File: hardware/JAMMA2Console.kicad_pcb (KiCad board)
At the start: 4 copper layers, 126 x 131.5 mm, 212 parts, among them J1 Conn_02x28_JAMMA, J10 Conn_02x03_Odd_Even, J11 Conn_02x05_Odd_Even, J12 Conn_01x03, J13 Conn_01x03, J2 DS1038-15FBNSiA74-0CC, J3 SCART-F, J4 DF1BZ-34DP-2.5DSA, J5 PJ-320D, J6 DS1037-15FNAKT74-0CC, J7 DS1037-15FNAKT74-0CC, J8 Phoenix PTS 1,5/4-5.0, J9 Molex 67503-1020, SW1 SW_Push, SW2 SW_Push, SW3 SW_Push, U1 USBLC6-2P6, U10 74LVC4245, U11 74LVC4245, U13 PAM8610, U14 PAM8610, U15 74HCT4053, U16 STM32F103VCT6, U2 LD1117-3.3, U3 74HCT4053, U4 74HCT86, U5 74HCT4053, U6 LM1881, U7 THS7375, U8 TL072, U9 74LVC4245, Y1 12MHz

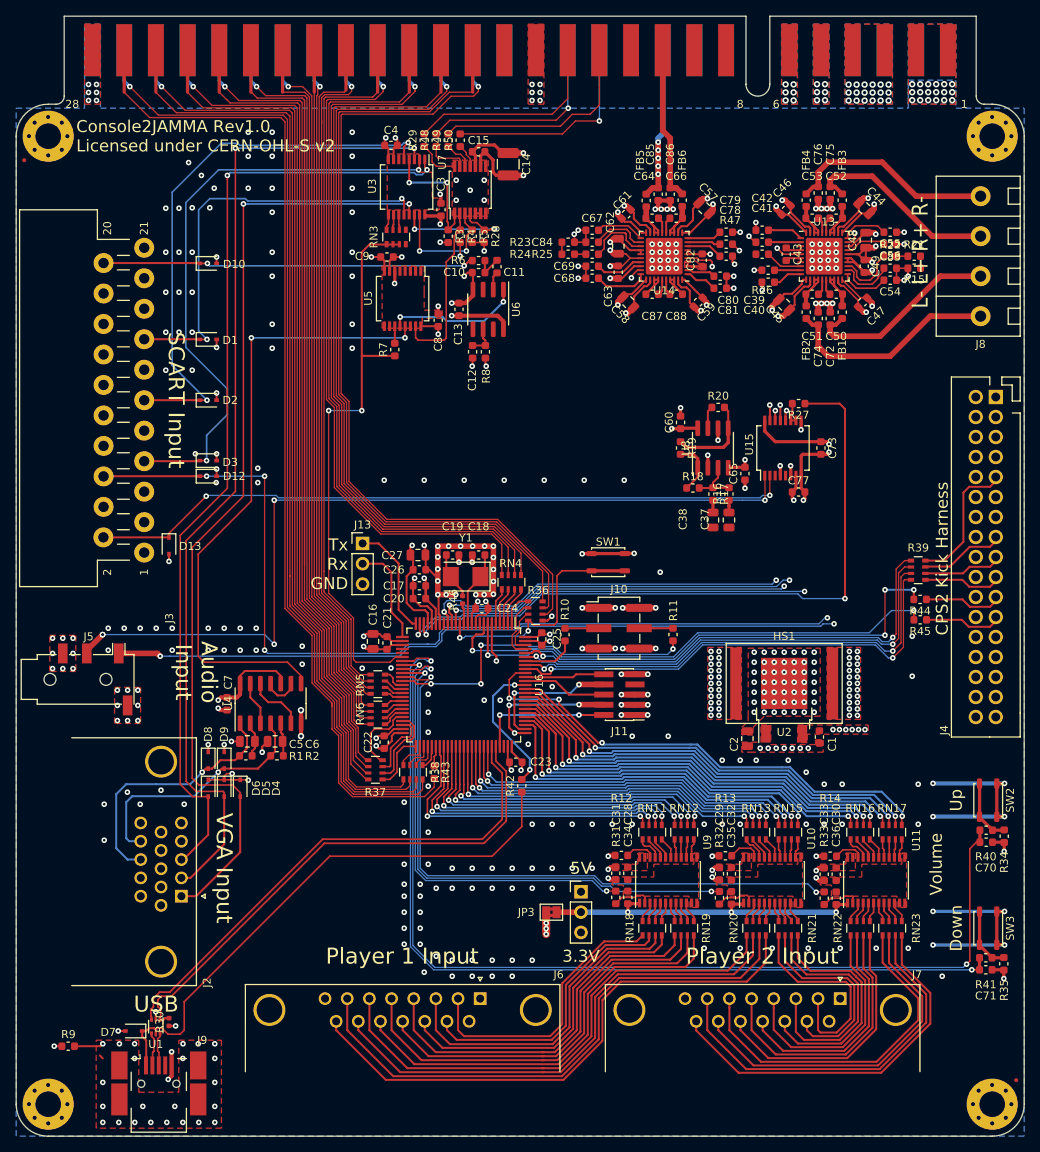
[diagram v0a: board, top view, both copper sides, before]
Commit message: Pushing work I did a few months ago and I forgot to push. Identified some mistakes which I'll fix in a future commit.
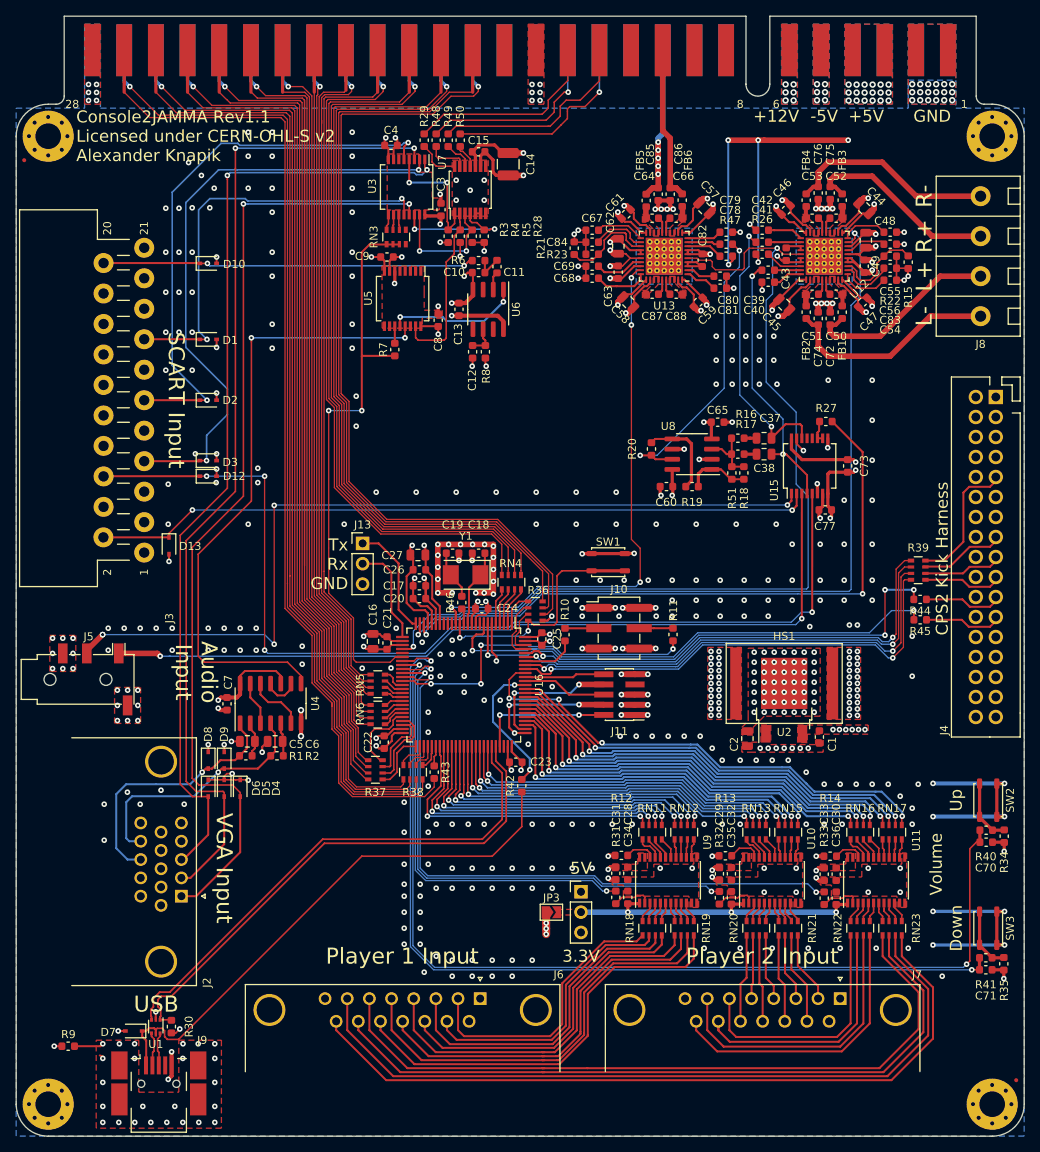
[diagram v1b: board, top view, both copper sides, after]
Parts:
- removed R24: 10K, Resistor_SMD:R_0603_1608Metric
- removed R25: 100K, Resistor_SMD:R_0603_1608Metric
- removed U14: PAM8610, Package_DFN_QFN:QFN-40-1EP_6x6mm_P0.5mm_EP4.6x4.6mm
- added R51: 10K, Resistor_SMD:R_0603_1608Metric, F.Cu at (125.5, 87.6)
- added U12: PAM8610, Console2JAMMA:QFN-40-1EP_6x6mm_P0.5mm_EP4.6x4.6mm_ThermalVias, F.Cu at (137.0, 60.5)
- C83, C84: value 200p -> 10n
- JP3: footprint Jumper:SolderJumper-2_P1.3mm_Bridged2Bar_Pad1.0x1.5mm -> Jumper:SolderJumper-2_P1.3mm_Open_TrianglePad1.0x1.5mm
- R15, R21, R23: value 10K -> 4K7
- R18: value 4K7 -> 10K
- R22: value 100K -> 4K7
- R30, R46: footprint Resistor_SMD:R_0402_1005Metric -> Resistor_SMD:R_0603_1608Metric
- U13: footprint Package_DFN_QFN:QFN-40-1EP_6x6mm_P0.5mm_EP4.6x4.6mm -> Console2JAMMA:QFN-40-1EP_6x6mm_P0.5mm_EP4.6x4.6mm_ThermalVias
- moved R21 42.5 mm to (105.8, 59.5), turned to 90 degrees
- moved U13 20.0 mm to (117.0, 60.5), turned to 180 degrees
- moved C37 11.1 mm to (129.5, 83.2), turned to 0 degrees
- moved C38 10.4 mm to (129.5, 85.2), turned to 0 degrees
- moved R20 9.83 mm to (115.4, 84.6), turned to 90 degrees
- moved C60 8.22 mm to (117.3, 89.3), turned to 180 degrees
- moved C65 7.28 mm to (123.7, 81.2), turned to 180 degrees
- moved R16 7.06 mm to (126.2, 83.2), turned to 0 degrees
- moved R18 6.63 mm to (127.0, 87.6), turned to 90 degrees
- moved R17 5.87 mm to (126.2, 85.2), turned to 0 degrees
- moved R19 5.03 mm to (120.5, 89.3), turned to 0 degrees
- moved R27 4.08 mm to (137.2, 81.2)
- moved C73 4.02 mm to (139.9, 86.7)
- moved C77 4.02 mm to (137.1, 92.2)
- moved U15 4.02 mm to (135.2, 86.7)
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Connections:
- net /UART_RX renamed /Digital I/O/UART_Rx
- net /UART_TX renamed /Digital I/O/UART_Tx
- C37 pad 2: /Audio/Audio_L -> /Audio/Audio_R
- C38 pad 2: /Audio/Audio_R -> /Audio/Audio_L
- JP3 pad 1: /VCC -> Net-(J6-Pad1)
- JP3 pad 2: Net-(J6-Pad1) -> /VCC
- R21 pad 2: Net-(R15-Pad1) -> GND
- R22 pad 1: Net-(R22-Pad1) -> Net-(R15-Pad1)
- R22 pad 2: Net-(R21-Pad1) -> GND
- R23 pad 1: Net-(R23-Pad1) -> Net-(R21-Pad1)
- R26 pad 2: +3V3 -> +5V
- R47 pad 2: +3V3 -> +5V
- RN20 pad 1: /P1_9 -> /P2_8
- RN20 pad 2: /P1_10 -> /P2_7
- RN20 pad 3: /P1_11 -> /P2_6
- RN20 pad 4: /P1_12 -> /P2_5
- RN21 pad 1: /P2_1 -> /P2_4
- RN21 pad 2: /P2_2 -> /P2_3
- RN21 pad 3: /P2_3 -> /P2_2
- RN21 pad 4: /P2_4 -> /P2_1
- RN22 pad 1: /P2_5 -> /P2_9
- RN22 pad 2: /P2_6 -> /P2_10
- RN22 pad 3: /P2_7 -> /P2_11
- RN22 pad 4: /P2_8 -> /P2_12
- RN23 pad 1: /P2_9 -> /P1_9
- RN23 pad 2: /P2_10 -> /P1_10
- RN23 pad 3: /P2_11 -> /P1_11
- RN23 pad 4: /P2_12 -> /P1_12
- U13 pad 1: Net-(C42-Pad1) -> Net-(C81-Pad1)
- U13 pad 10: Net-(C40-Pad1) -> Net-(C79-Pad1)
- U13 pad 13: Net-(C51-Pad2) -> Net-(C66-Pad2)
- U13 pad 14: Net-(C51-Pad2) -> Net-(C66-Pad2)
- U13 pad 15: Net-(C51-Pad1) -> Net-(C66-Pad1)
- U13 pad 16: Net-(C50-Pad2) -> Net-(C64-Pad2)
- U13 pad 17: Net-(C50-Pad1) -> Net-(C64-Pad1)
- U13 pad 18: Net-(C50-Pad1) -> Net-(C64-Pad1)
- U13 pad 2: Net-(C41-Pad1) -> Net-(C80-Pad1)
- U13 pad 21: Net-(C54-Pad2) -> Net-(C67-Pad2)
- U13 pad 22: Net-(C83-Pad1) -> Net-(C84-Pad1)
- U13 pad 23: Net-(R22-Pad1) -> Net-(R21-Pad1)
- U13 pad 27: Net-(C56-Pad2) -> Net-(C69-Pad2)
- U13 pad 29: (no net) -> /~Mono_Shutdown~
- U13 pad 3: Net-(C43-Pad1) -> Net-(C82-Pad1)
- U13 pad 30: Net-(C55-Pad2) -> Net-(C68-Pad2)
- U13 pad 33: Net-(C52-Pad1) -> Net-(C87-Pad1)
- U13 pad 34: Net-(C52-Pad1) -> Net-(C87-Pad1)
- U13 pad 35: Net-(C52-Pad2) -> Net-(C87-Pad2)
- U13 pad 36: Net-(C53-Pad1) -> Net-(C88-Pad1)
- U13 pad 37: Net-(C53-Pad2) -> Net-(C88-Pad2)
- U13 pad 38: Net-(C53-Pad2) -> Net-(C88-Pad2)
- U13 pad 4: Net-(C43-Pad1) -> Net-(C82-Pad1)
- U13 pad 41: (no net) -> Net-(U13-Pad41)
- U13 pad 8: Net-(R26-Pad1) -> Net-(R47-Pad1)
- U13 pad 9: Net-(C39-Pad1) -> Net-(C78-Pad1)
- U15 pad 12: /SCART_Audio_L -> (no net)
- U15 pad 13: /EXT_Audio_L -> (no net)
- U15 pad 15: /Audio/Audio_L -> GND
- U15 pad 3: (no net) -> /EXT_Audio_L
- U15 pad 4: GND -> /Audio/Audio_L
- U15 pad 5: (no net) -> /SCART_Audio_L
- U16 pad 15: (no net) -> /~Mono_Shutdown~
- U16 pad 24: (no net) -> /~Stereo_Shutdown~
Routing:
- net /Volume: track 7.10 -> 118.2 mm
- net /~Stereo_Shutdown~: track 0.00 -> 104.9 mm, vias 0 -> 2
- net /~Mono_Shutdown~: track 0.00 -> 68.5 mm, vias 0 -> 4
- net /Audio_Select_~Mono~_Stereo: track 52.0 -> 0.00 mm, vias 2 -> 0
- net Net-(U16-Pad16): track 46.6 -> 0.00 mm, vias 2 -> 0
- net Net-(U16-Pad17): track 46.0 -> 0.00 mm, vias 2 -> 0
- net Net-(U16-Pad15): track 44.0 -> 0.00 mm, vias 2 -> 0
- net +5V: track 148.4 -> 186.2 mm, vias 31 -> 36
- net /Audio/Audio_Mono: track 4.00 -> 37.4 mm, vias 1 -> 2
- net /Audio/Audio_R: track 2.41 -> 34.7 mm
- net /Audio/Audio_L: track 2.90 -> 33.2 mm
- net /P1_9: track 64.4 -> 90.4 mm
- net /P2_7: track 33.7 -> 7.97 mm
- net /P1_10: track 64.4 -> 90.1 mm
- net /P1_11: track 69.9 -> 95.3 mm
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- added copper zone on In2.Cu, net +12V
- added copper zone on F.Cu, net /VCC
- added copper zone on F.Cu, net Net-(C50-Pad1)
- added copper zone on F.Cu, net Net-(C51-Pad2)
- added copper zone on F.Cu, net Net-(C52-Pad1)
- added copper zone on F.Cu, net Net-(C53-Pad2)
- added copper zone on F.Cu, net Net-(C64-Pad1)
- added copper zone on F.Cu, net Net-(C66-Pad2)
- added copper zone on F.Cu, net Net-(C87-Pad1)
- added copper zone on F.Cu, net Net-(C88-Pad2)
- added copper zone on In2.Cu, net Net-(J9-Pad6)
- added copper zone on B.Cu, net Net-(U12-Pad41)
- added copper zone on In2.Cu, net Net-(U12-Pad41)
- added copper zone on B.Cu, net Net-(U13-Pad41)
- added copper zone on In2.Cu, net Net-(U13-Pad41)
- removed copper zone on F.Cu, net Net-(C82-Pad1)
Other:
- rule trace_min: 0.1524 -> 0.152
- board text added: "+12V"
- board text added: "+5V"
- board text added: "-5V"
- board text added: "Console2JAMMA Rev1.1 Licensed under CERN-OHL-S v2 Alexander Knapik"
- board text added: "GND"
- board text added: "L+"
- board text added: "L-"
- board text added: "R+"
- board text added: "R-"
- board text removed: "Console2JAMMA Rev1.0 Licensed under CERN-OHL-S v2"
- board text removed: "L- L+ R+ R-"
